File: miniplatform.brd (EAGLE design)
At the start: 40 x 80 mm, 9 parts

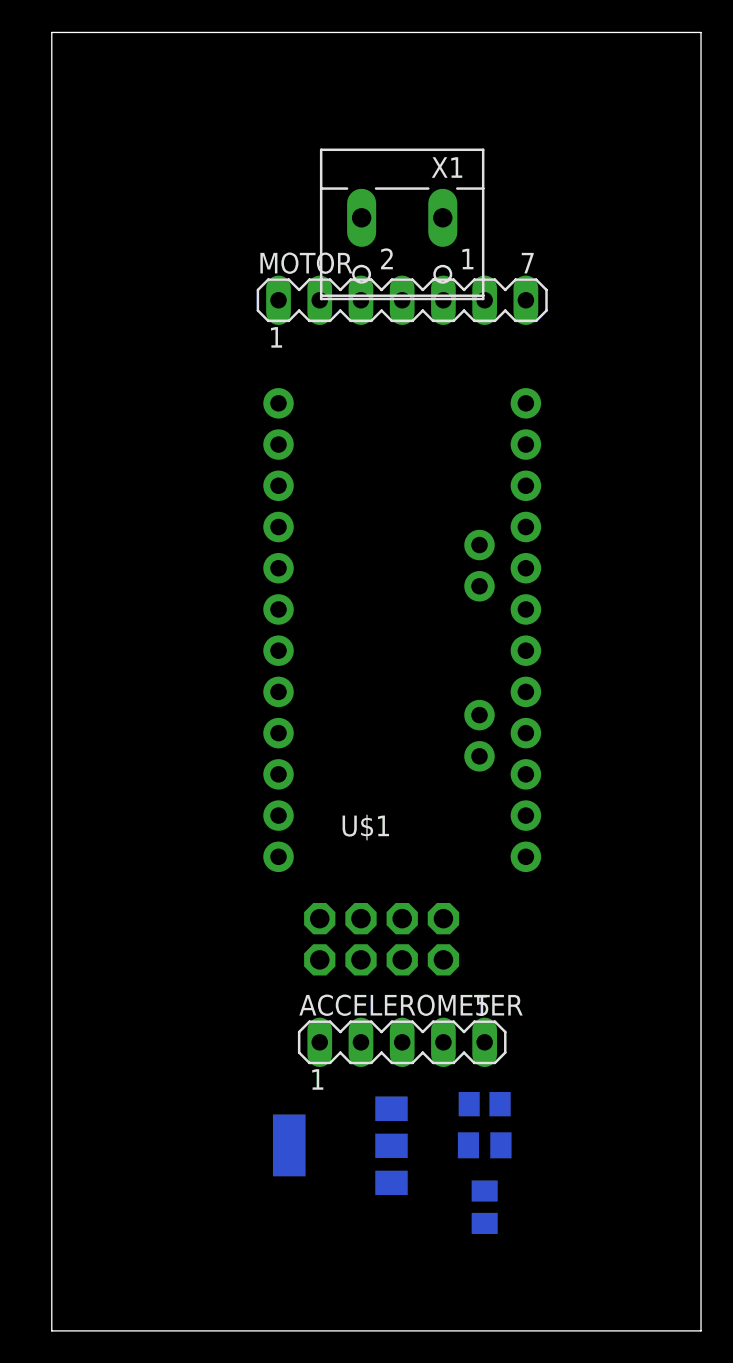
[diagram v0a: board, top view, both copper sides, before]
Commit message: Tuned layout.
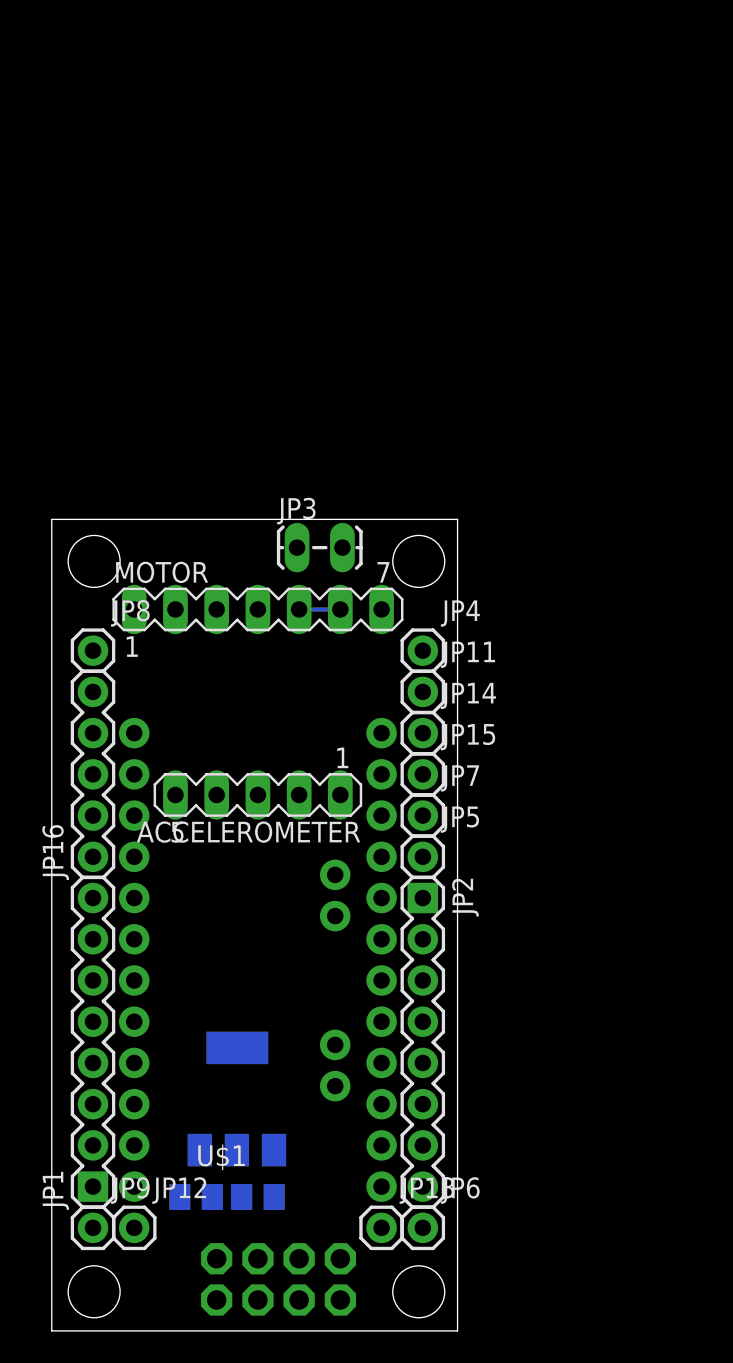
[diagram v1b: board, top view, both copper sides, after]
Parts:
- removed R1: 1k, rcl:R0805
- removed X1: (no value), con-wago-500:W237-102
- added JP1, JP2: (no value), SparkFun:1X08
- added JP11, JP12, JP13, JP14, JP15, JP4, JP5, JP6, JP7, JP8, JP9: M01PTH, SparkFun:1X01
- added JP16: (no value), SparkFun:1X05
- added JP3: (no value), SparkFun:1X02_LOCK_LONGPADS
- moved U$2 23.5 mm to (17.8, 1.91), turned to 0 degrees
- moved U$1 22.2 mm to (12.7, 24.1)
- moved MOTOR 21.0 mm to (12.7, 44.5)
- moved C7 17.8 mm to (8.89, 8.26), turned to 0 degrees
- moved ACCELEROMETER 17.6 mm to (12.7, 33.0), turned to 180 degrees
- moved C12 14.3 mm to (12.7, 8.26)
- moved 3.3V_REG 6.96 mm to (11.4, 14.3), turned to 0 degrees
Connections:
- removed net ANALOG_6: U$1.A7
- removed net IO1: U$1.10
- removed net LATCH: MOTOR.2, U$1.7
- removed net MOTOR_SELECT: MOTOR.4, U$1.5
- new net ANALOG_3: U$1.A6
- new net MOTOR_CLOCK: JP1.3, MOTOR.3, U$1.10
- new net MOTOR_DATA: JP1.8, MOTOR.1, U$1.5
- new net MOTOR_LATCH: JP1.6, MOTOR.2, U$1.7
- net +3V3: now also JP6.1, JP9.1; no longer R1.2
- net +5V: now also JP16.5, JP5.1, MOTOR.4
- net ACCEL_Z: now also U$1.A7; no longer U$1.A6
- net ANALOG_1: now also JP2.2
- net ANALOG_2: now also JP2.1
- net CLOCK: now also JP2.5; no longer MOTOR.3
- net GND: now also JP12.1, JP13.1, JP14.1, JP15.1, JP16.1, JP3.1, JP7.1, JP8.1; no longer R1.1, X1.2
- net IO2: now also JP1.2
- net MISO: now also JP2.6
- net MOSI: now also JP2.7; no longer MOTOR.1
- net PWM1: now also JP1.7
- net PWM2: now also JP1.5
- net PWM3: now also JP1.4
- net PWM4: now also JP1.1
- net PWM5: now also JP2.8
- net RADIO_CE: now also JP2.3
- net RADIO_CSN: now also JP2.4
- net RESET: now also JP16.2
- net TXI: now also JP16.3
- net TXO: now also JP16.4
- net VCC: now also JP11.1, JP3.2, JP4.1; no longer X1.1
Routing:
- net GND: track 0.00 -> 2.54 mm
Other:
- board size 40 x 80 mm -> 25 x 50 mm
